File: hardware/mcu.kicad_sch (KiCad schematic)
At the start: 22 parts, among them J301 TagConnect, J302 USER CONN., SW301 USER, U301 STM32G431, U302 SN65HVD230, Y301 12MHz

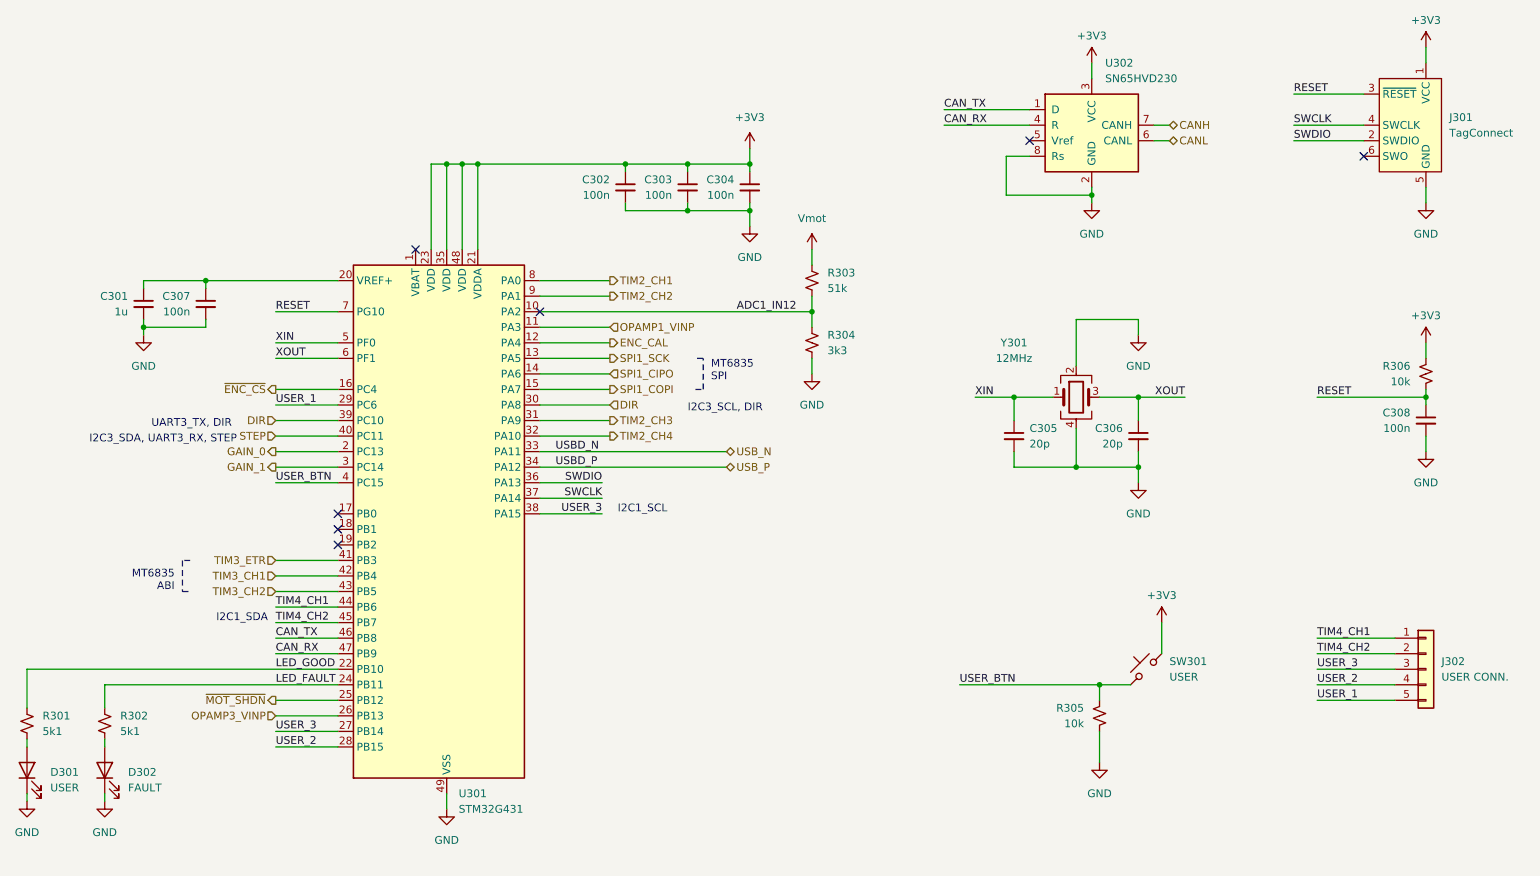
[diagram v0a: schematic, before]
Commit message: clean erc drc, pack sym, footprints into standalone lib
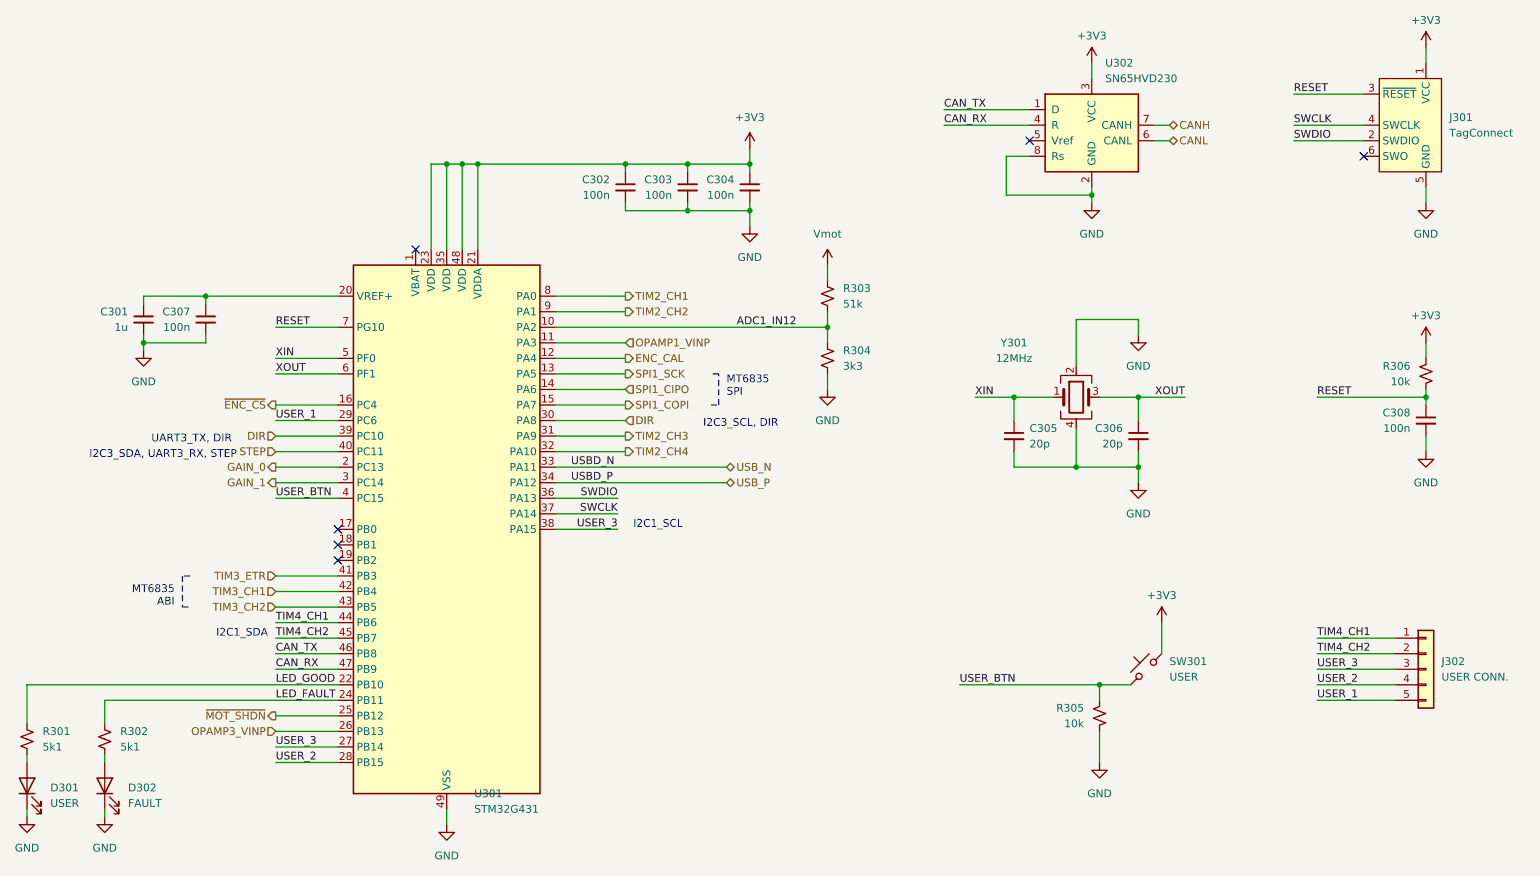
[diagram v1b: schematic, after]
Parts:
- C301, C302, C303, C304, C305, C306, C307, C308: footprint Capacitor_SMD:C_0402_1005Metric -> lemon-pepper-footprints:C_0402_1005Metric; symbol Device:C_Small -> lemon-pepper-symbols:C_Small
- D301, D302: footprint Diode_SMD:D_0603_1608Metric -> lemon-pepper-footprints:D_0603_1608Metric; symbol Device:LED -> lemon-pepper-symbols:LED
- J301: symbol Connector:Conn_ARM_SWD_TagConnect_TC2030-NL -> lemon-pepper-symbols:Conn_ARM_SWD_TagConnect_TC2030-NL
- J302: footprint mechanical:PinHeader_1x05_P1.27mm_SMD -> lemon-pepper-footprints:PinHeader_1x05_P1.27mm_SMD; symbol Connector_Generic:Conn_01x05 -> lemon-pepper-symbols:Conn_01x05
- R301, R302, R303, R304, R305, R306: footprint Resistor_SMD:R_0402_1005Metric -> lemon-pepper-footprints:R_0402_1005Metric; symbol Device:R_Small_US -> lemon-pepper-symbols:R_Small_US
- SW301: footprint Button_Switch_SMD:SW_SPST_B3U-3000P -> lemon-pepper-footprints:SW_SPST_B3U-3000P; symbol Switch:SW_Push_45deg -> lemon-pepper-symbols:SW_Push_45deg
- U301: footprint Package_DFN_QFN:QFN-48-1EP_7x7mm_P0.5mm_EP5.6x5.6mm -> lemon-pepper-footprints:QFN-48-1EP_7x7mm_P0.5mm_EP5.6x5.6mm; symbol MCU_ST_STM32G4:STM32G431CBUx -> lemon-pepper-symbols:STM32G431CBUx
- U302: footprint Package_SO:SOIC-8_3.9x4.9mm_P1.27mm -> lemon-pepper-footprints:SOIC-8_3.9x4.9mm_P1.27mm; symbol Interface_CAN_LIN:SN65HVD230 -> lemon-pepper-symbols:SN65HVD230
- Y301: footprint Crystal:Crystal_SMD_3225-4Pin_3.2x2.5mm -> lemon-pepper-footprints:Crystal_SMD_3225-4Pin_3.2x2.5mm; symbol Device:Crystal_GND24 -> lemon-pepper-symbols:Crystal_GND24
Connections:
- no-connect marks 7 -> 6
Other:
- moved on the sheet: C301, C307, D301, D302, R301, R302, R303, R304, U301
